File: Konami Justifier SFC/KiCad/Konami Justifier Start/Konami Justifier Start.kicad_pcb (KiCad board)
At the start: 4 copper layers, 15.2 x 15.4 mm, 7 parts, among them SW1 SW_Push_Open

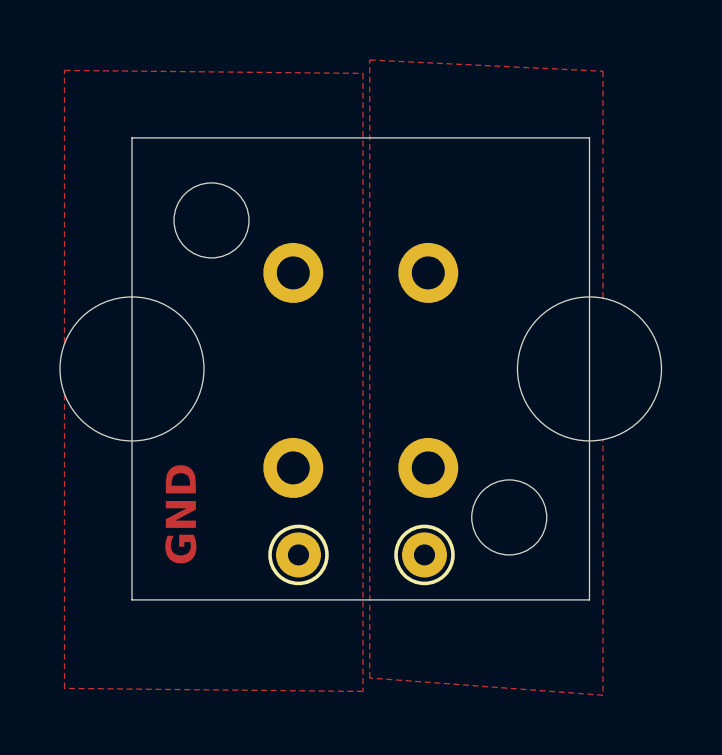
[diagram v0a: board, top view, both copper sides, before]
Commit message: Add files via upload
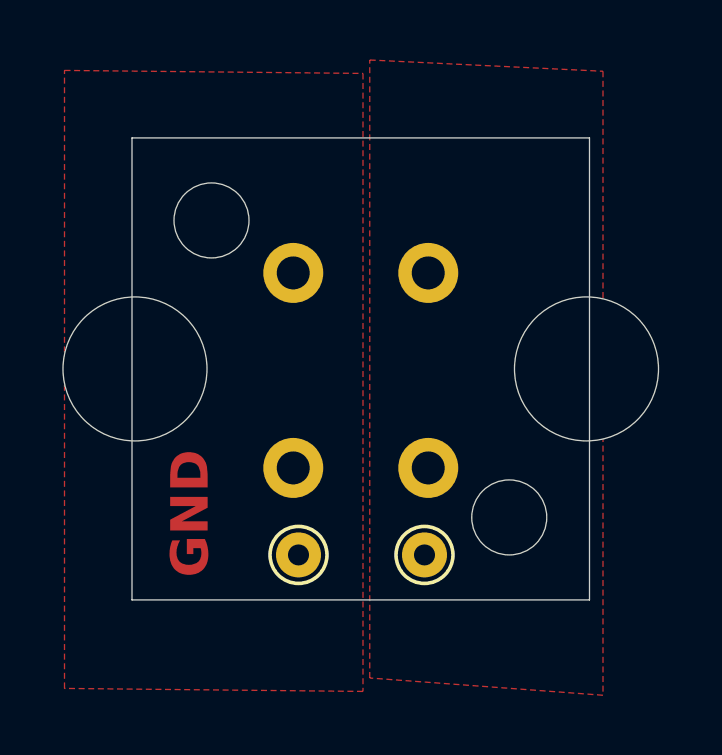
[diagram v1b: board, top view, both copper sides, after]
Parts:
- moved REF** 0.10 mm to (151.4, 99.2)
- moved REF** 0.10 mm to (136.3, 99.2)
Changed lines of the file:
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@@
 		(tenting front back)
 		(pcbplotparams
-			(layerselection 0x00000000_00000000_55555555_5755f5ff)
+			(layerselection 0x00000000_00000000_55555555_5755f5af)
 			(plot_on_all_layers_selection 0x00000000_00000000_00000000_00000000)
 			(disableapertmacros no)
@@
 			(outputformat 1)
 			(mirror no)
-			(drillshape 1)
+			(drillshape 0)
 			(scaleselection 1)
-			(outputdirectory "")
+			(outputdirectory "C:/Users/ifreund/Documents/Konami Justifier Start/Gerbers/")
 		)
 	)
@@
 		(locked yes)
 		(layer "F.Cu")
-		(at 151.5 99.199838 90)
+		(at 151.4 99.199838 90)
 		(descr "Mounting Hole 5.3mm, M5, no annular, generated by kicad-footprint-generator mountinghole.py")
 		(tags "mountinghole M5")
@@
 		(locked yes)
 		(layer "F.Cu")
-		(at 136.25 99.2 -90)
+		(at 136.35 99.2 -90)
 		(descr "Mounting Hole 5.3mm, M5, no annular, generated by kicad-footprint-generator mountinghole.py")
 		(tags "mountinghole M5")
@@
 	)
 	(gr_text "GND"
-		(at 138.5 105.75 90)
+		(at 138.925 106.15 90)
 		(layer "F.Cu" knockout)
 		(effects
 			(font
-				(size 1 1)
-				(thickness 0.2)
+				(size 1.25 1.25)
+				(thickness 0.25)
 				(bold yes)
 			)
